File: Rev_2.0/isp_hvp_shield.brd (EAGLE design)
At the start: 50 x 53 mm, 26 parts, among them IC1 ATtiny13/15/25/45/85, IC2 ATtiny24/44/84, IC3 TINY26/261/461/861, IC4 ATtiny2313/4313, IC5 ATMEGA328, IC6 74HCT595D, IC7 MAX662A, Q1 BC858BSMD

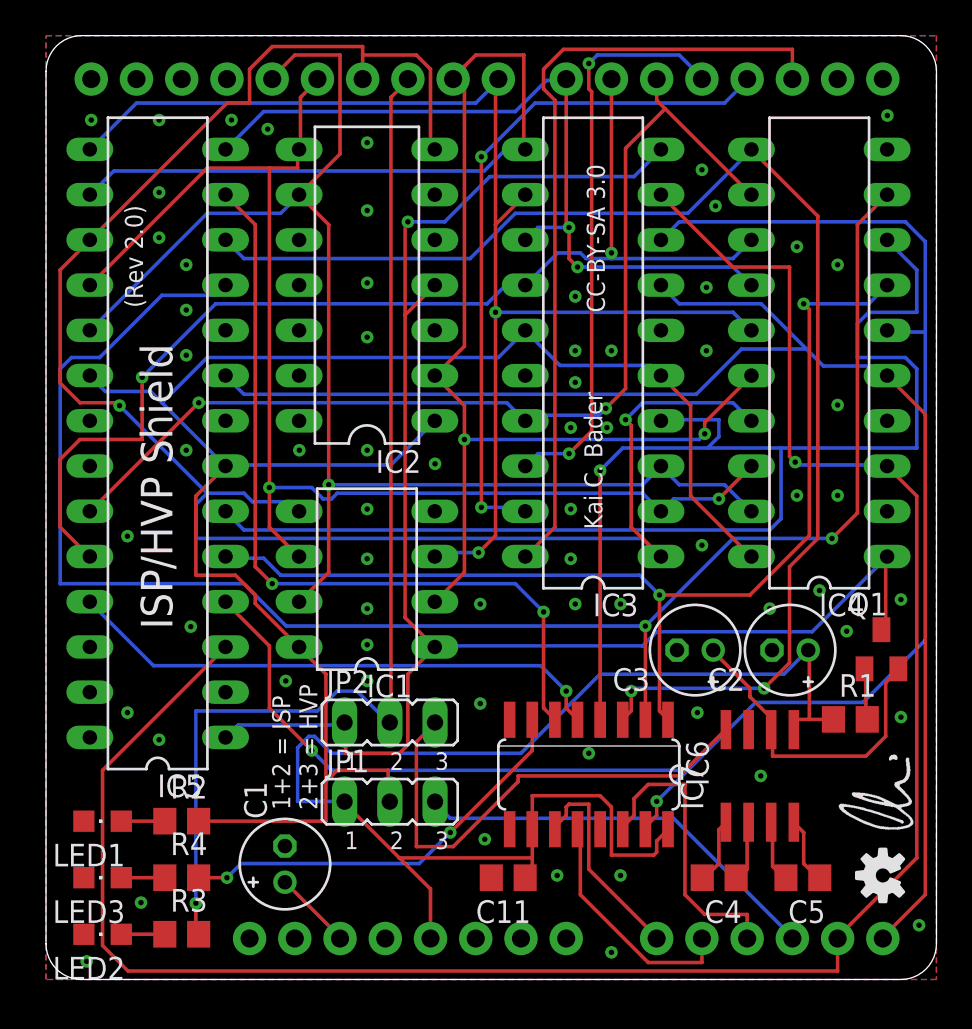
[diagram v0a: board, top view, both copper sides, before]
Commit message: More cleaning...
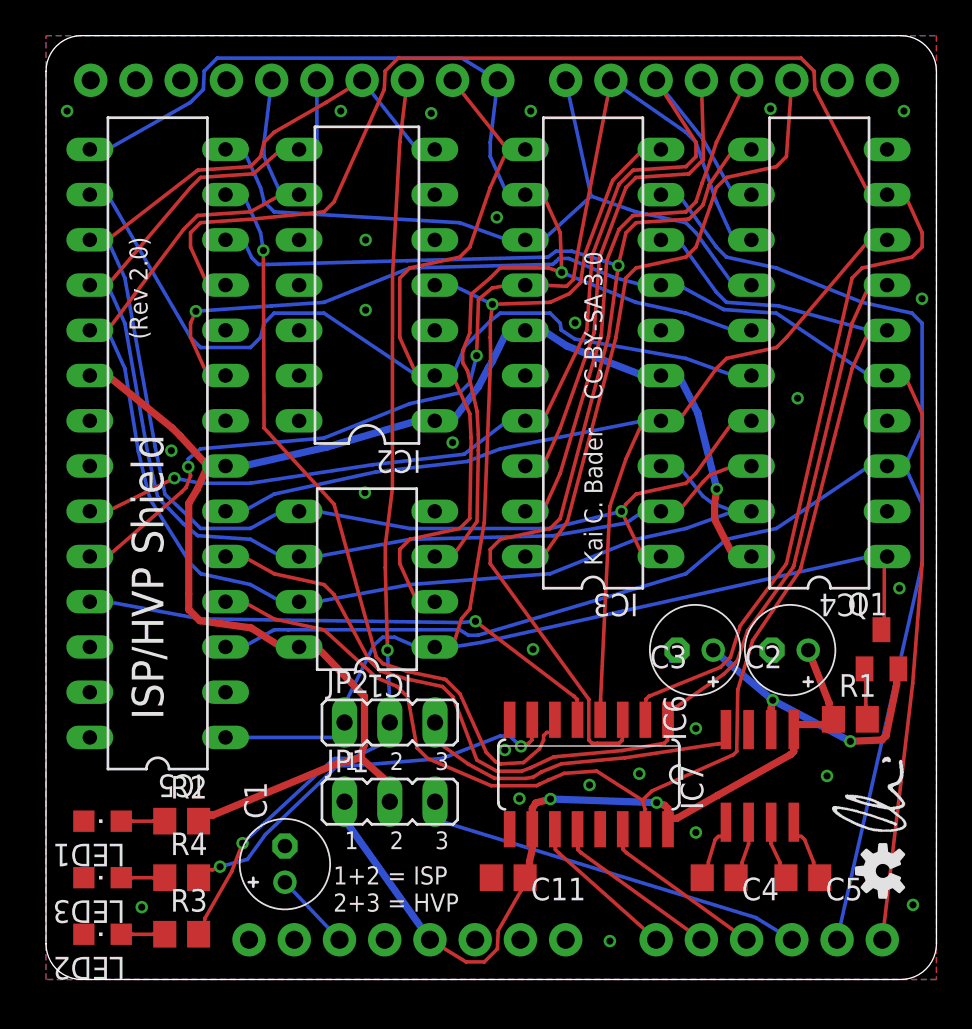
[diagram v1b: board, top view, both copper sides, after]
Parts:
- removed U$1: (no value), kaibader:OSHW-LOGO-S
- removed U$3: (no value), kaibader:KAI-LOGO-M
- added E$1: (no value), kaibader:KAI-LOGO-M
- added E$2: (no value), kaibader:OSHW-LOGO-S
- PINS: value UNO_R3_SHIELDV1 -> (none)
- moved PINS 0.08 mm to (-7.65, 53.0)
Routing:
- net Q4: track 91.6 -> 60.6 mm, vias 1 -> 0
- net VCC: track 77.6 -> 47.6 mm, vias 0 -> 2
- net A4: track 117.6 -> 94.5 mm, vias 1 -> 0
- net D11_MOSI: track 102.4 -> 80.4 mm, vias 2 -> 1
- net Q0: track 92.9 -> 77.1 mm, vias 2 -> 0
- net +5V: track 103.3 -> 88.1 mm, vias 0 -> 1
- net D2: track 44.4 -> 34.2 mm
- net D3: track 39.0 -> 29.8 mm, vias 2 -> 0
- net N$1: track 27.7 -> 18.8 mm
- net D10_RESET: track 93.3 -> 85.0 mm
- net D10: track 61.3 -> 53.2 mm, vias 1 -> 2
- net A2_SER: track 16.7 -> 9.73 mm
- net Q3: track 74.9 -> 69.2 mm, vias 2 -> 1
- net D4: track 32.4 -> 26.8 mm, vias 2 -> 0
- net A1_RCK: track 13.5 -> 9.73 mm
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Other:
- board text added: "Kai C. Bader CC-BY-SA 3.0"
- board text removed: "CC-BY-SA 3.0"
- board text removed: "Kai C. Bader"
